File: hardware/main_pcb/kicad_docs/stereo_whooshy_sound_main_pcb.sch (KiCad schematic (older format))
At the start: 2 parts, among them J10 IO_B, J9 IO_A

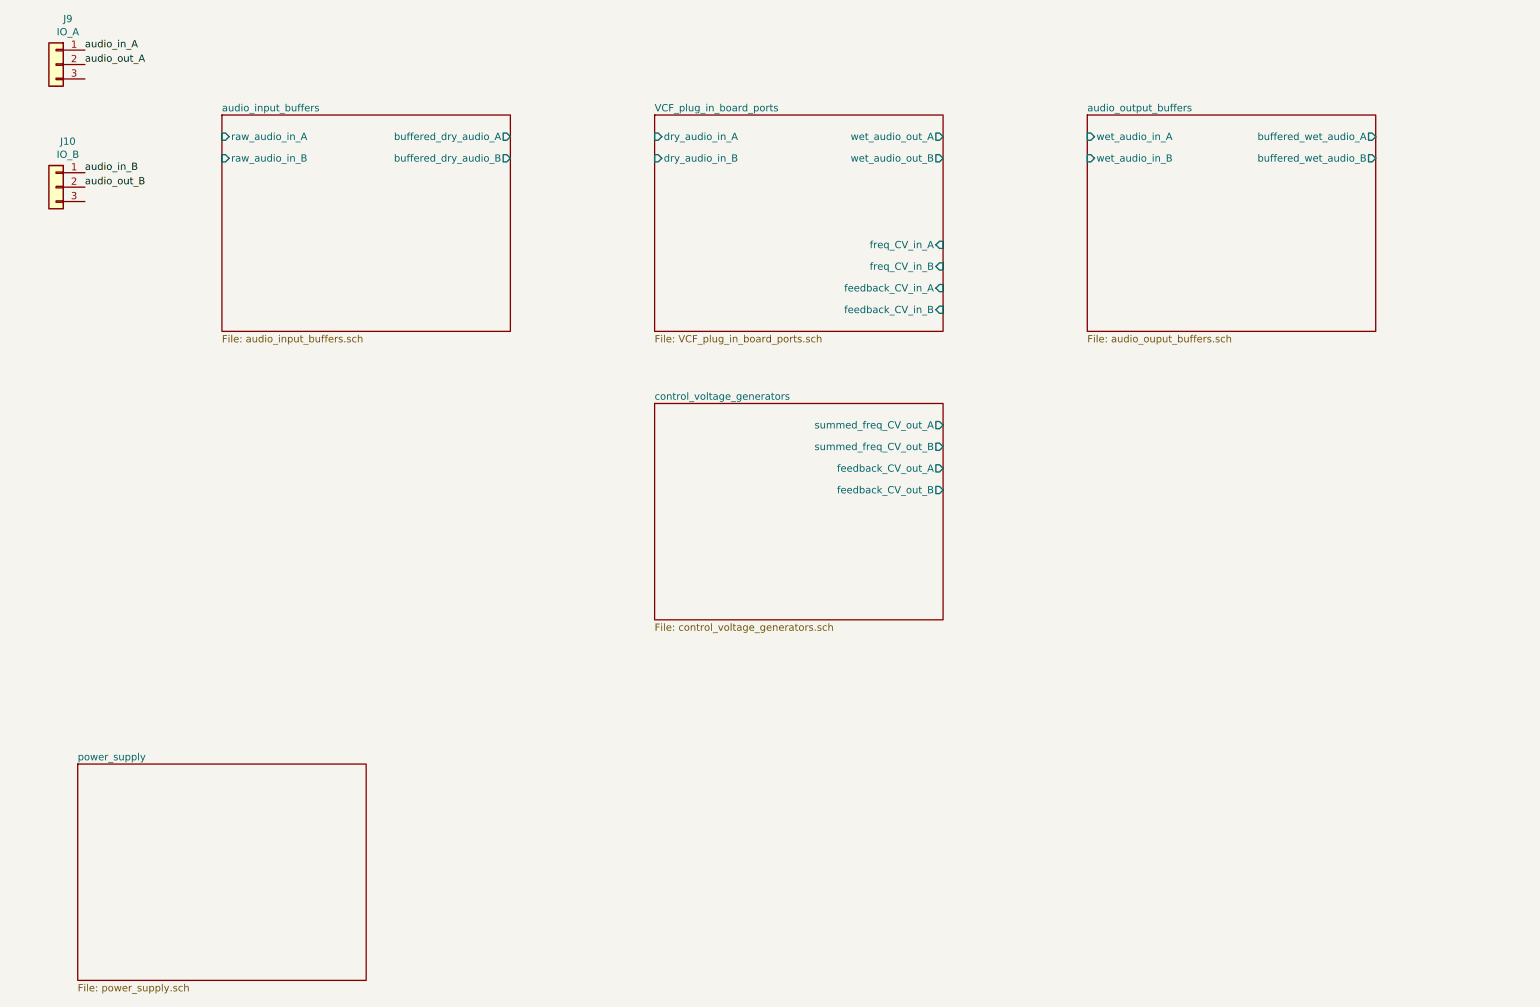
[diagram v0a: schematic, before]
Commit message: progress on pcb layout
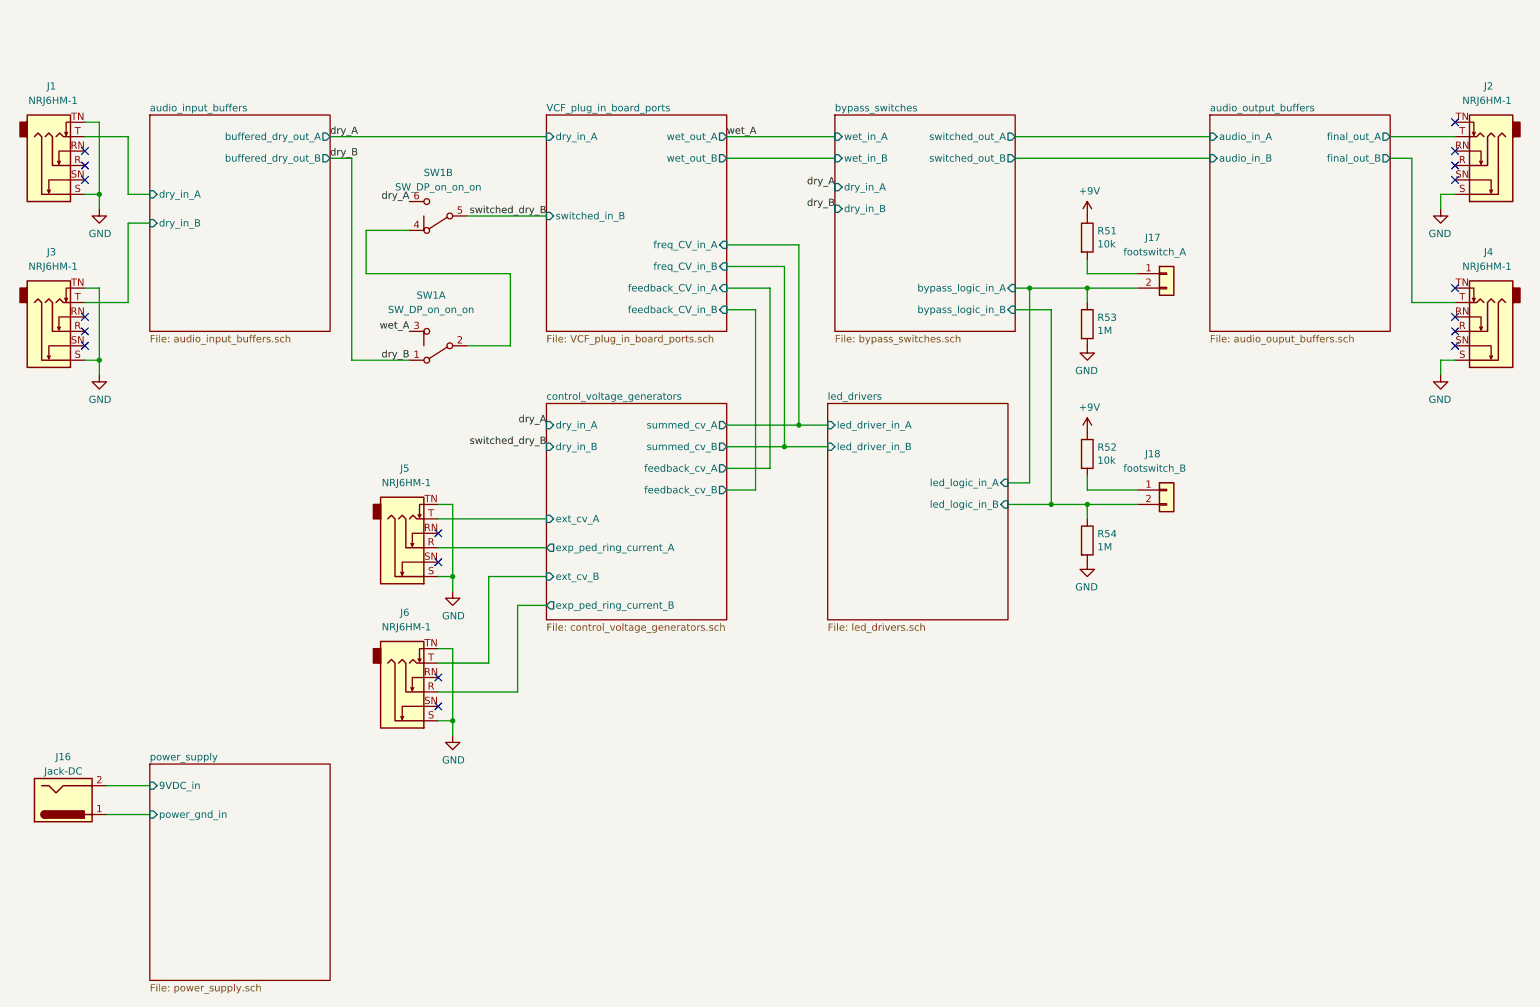
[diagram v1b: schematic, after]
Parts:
- removed J10: IO_B, Connector_PinHeader_2.54mm:PinHeader_1x03_P2.54mm_Vertical, symbol Connector_Generic:Conn_01x03
- removed J9: IO_A, Connector_PinHeader_2.54mm:PinHeader_1x03_P2.54mm_Vertical, symbol Connector_Generic:Conn_01x03
- added J1, J2, J3, J4, J5, J6: NRJ6HM-1, Connector_Audio:Jack_6.35mm_Neutrik_NRJ6HM-1_Horizontal, symbol Connector:AudioJack3_Switch
- added J16: Jack-DC, Connector_BarrelJack:BarrelJack_CUI_PJ-063AH_Horizontal, symbol Connector:Jack-DC
- added J17: footswitch_A, Connector_PinHeader_2.54mm:PinHeader_1x02_P2.54mm_Vertical, symbol Connector_Generic:Conn_01x02
- added J18: footswitch_B, Connector_PinHeader_2.54mm:PinHeader_1x02_P2.54mm_Vertical, symbol Connector_Generic:Conn_01x02
- added R51, R52: 10k, Resistor_SMD:R_0603_1608Metric, symbol Device:R
- added R53, R54: 1M, Resistor_SMD:R_0603_1608Metric, symbol Device:R
- added SW1: SW_DP_on_on_on, custom_footprints:DPDT_mini_toggle, symbol custom_components:SW_DP_on_on_on
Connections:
- new net: SW1.2 (B), SW1.4 (A)
- new net: J18.1 (Pin_1), R52.2
- new net: J17.1 (Pin_1), R51.2
- new net +9V: R51.1, R52.1
- new net GND: J1.S, J1.TN, J2.S, J3.S, J3.TN, J4.S, J5.S, J5.TN, J6.S, J6.TN, R53.2, R54.2
- new net audio_input_buffers/dry_in_A: J1.T
- new net audio_input_buffers/dry_in_B: J3.T
- new net audio_output_buffers/final_out_A: J2.T
- new net audio_output_buffers/final_out_B: J4.T
- new net bypass_switches/bypass_logic_in_A: J17.2 (Pin_2), R53.1
- new net bypass_switches/bypass_logic_in_B: J18.2 (Pin_2), R54.1
- new net control_voltage_generators/exp_ped_ring_current_A: J5.R
- new net control_voltage_generators/exp_ped_ring_current_B: J6.R
- new net control_voltage_generators/ext_cv_A: J5.T
- new net control_voltage_generators/ext_cv_B: J6.T
- new net dry_A: SW1.6 (C)
- new net dry_B: SW1.1 (A)
- new net power_supply/9VDC_in: J16.2
- new net power_supply/power_gnd_in: J16.1
- new net switched_dry_B: SW1.5 (B)
- new net wet_A: SW1.3 (C)
- no-connect marks 0 -> 18
